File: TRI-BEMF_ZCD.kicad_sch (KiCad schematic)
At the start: 22 parts, among them U2 LMV321, U3 LMV321, U4 LMV321

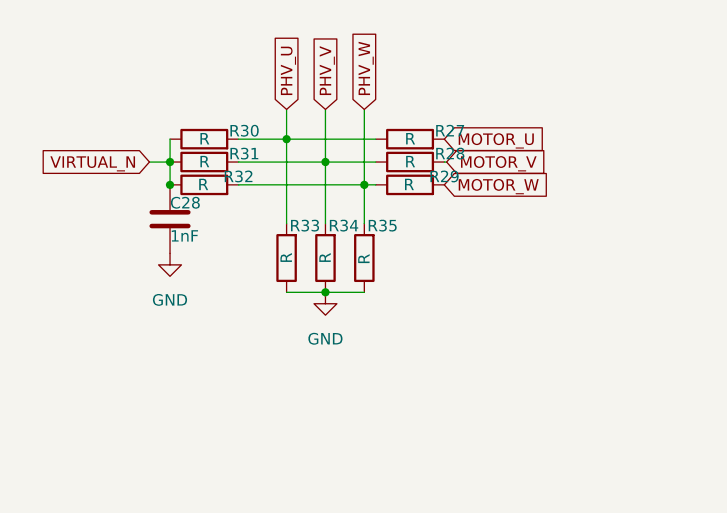
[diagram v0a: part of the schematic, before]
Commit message: v0.02
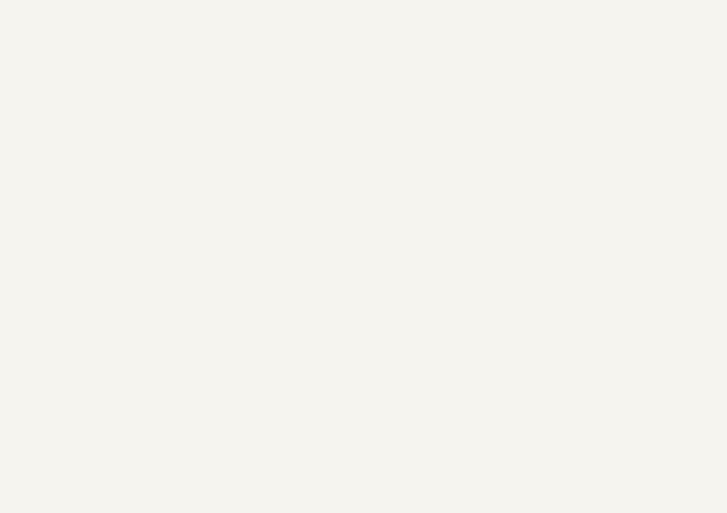
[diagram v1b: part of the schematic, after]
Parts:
- removed C28: 1nF, Capacitor_SMD:C_1206_3216Metric, symbol Device:C
- removed R27, R28, R29, R30, R31, R32, R33, R34, R35: R, Resistor_SMD:R_1206_3216Metric, symbol Device:R
